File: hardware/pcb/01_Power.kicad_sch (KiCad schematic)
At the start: 19 parts, among them J1 USB_C_Receptacle_USB2.0_16P, U1 TLV62569DBV, U5 TLV62569DBV

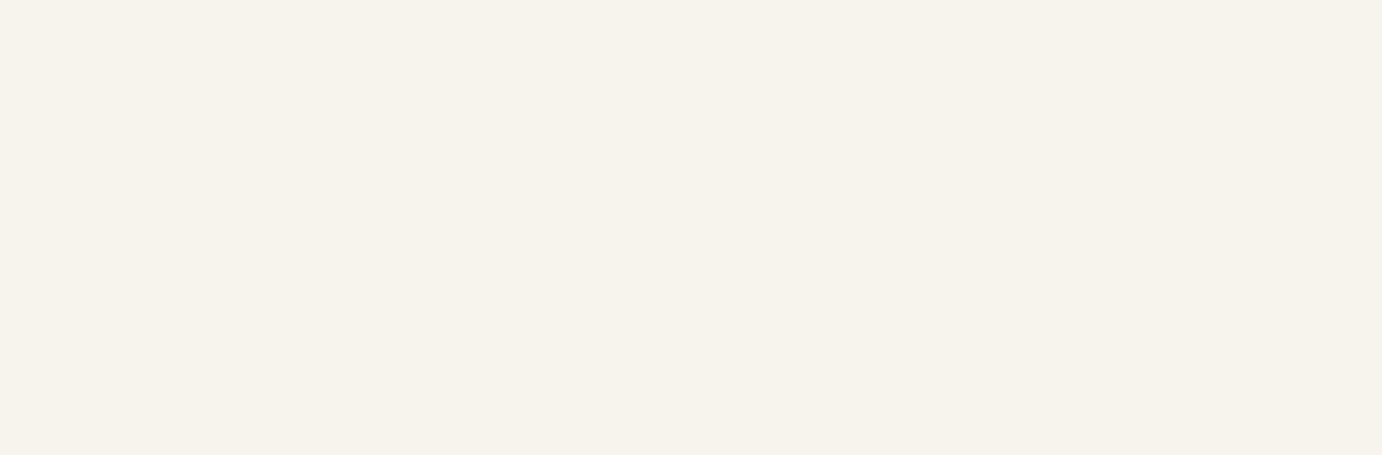
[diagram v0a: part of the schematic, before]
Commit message: feat: the power circuit is fully made with all rails
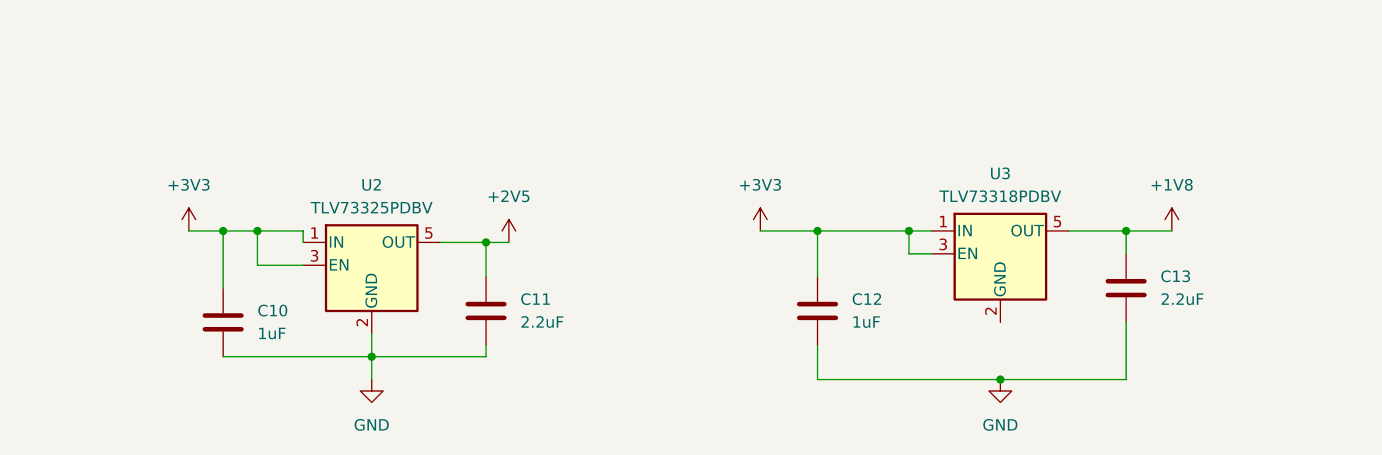
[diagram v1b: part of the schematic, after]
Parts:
- added C10, C12: 1uF, symbol Device:C
- added C11, C13: 2.2uF, symbol Device:C
- added U2: TLV73325PDBV, Package_TO_SOT_SMD:SOT-23-5, symbol Regulator_Linear:TLV73325PDBV
- added U3: TLV73318PDBV, Package_TO_SOT_SMD:SOT-23-5, symbol Regulator_Linear:TLV73318PDBV
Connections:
- net +3V3: now also C10.1, C12.1, U2.1 (IN), U2.3 (EN), U3.1 (IN), U3.3 (EN)
- net GND: now also C10.2, C11.2, C12.2, C13.2, U2.2 (GND)
- new net +1V8: C13.1, U3.5 (OUT)
- new net +2V5: C11.1, U2.5 (OUT)
